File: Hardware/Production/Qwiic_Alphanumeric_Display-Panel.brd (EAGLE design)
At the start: 240.5 x 155.4 mm, 1080 parts, among them J11 Vertical Qwiic Connector, J12 Vertical Qwiic Connector, J14 Vertical Qwiic Connector, J15 Vertical Qwiic Connector, J17 Vertical Qwiic Connector, J18 Vertical Qwiic Connector, J2 Vertical Qwiic Connector, J20 Vertical Qwiic Connector, J21 Vertical Qwiic Connector, J23 Vertical Qwiic Connector, J24 Vertical Qwiic Connector, J26 Vertical Qwiic Connector, J27 Vertical Qwiic Connector, J29 Vertical Qwiic Connector, J30 Vertical Qwiic Connector, J32 Vertical Qwiic Connector, J33 Vertical Qwiic Connector, J35 Vertical Qwiic Connector, J36 Vertical Qwiic Connector, J38 Vertical Qwiic Connector, J39 Vertical Qwiic Connector, J4 Vertical Qwiic Connector, J41 Vertical Qwiic Connector, J42 Vertical Qwiic Connector, J44 Vertical Qwiic Connector, J45 Vertical Qwiic Connector, J47 Vertical Qwiic Connector, J48 Vertical Qwiic Connector, J5 Vertical Qwiic Connector, J50 Vertical Qwiic Connector, J51 Vertical Qwiic Connector, J53 Vertical Qwiic Connector, J54 Vertical Qwiic Connector, J56 Vertical Qwiic Connector, J57 Vertical Qwiic Connector, J59 Vertical Qwiic Connector, J6 Vertical Qwiic Connector, J60 Vertical Qwiic Connector, J62 Vertical Qwiic Connector, J63 Vertical Qwiic Connector, J65 Vertical Qwiic Connector, J66 Vertical Qwiic Connector, J68 Vertical Qwiic Connector, J69 Vertical Qwiic Connector, J71 Vertical Qwiic Connector, J72 Vertical Qwiic Connector, J74 Vertical Qwiic Connector, J75 Vertical Qwiic Connector, J8 Vertical Qwiic Connector, J9 Vertical Qwiic Connector

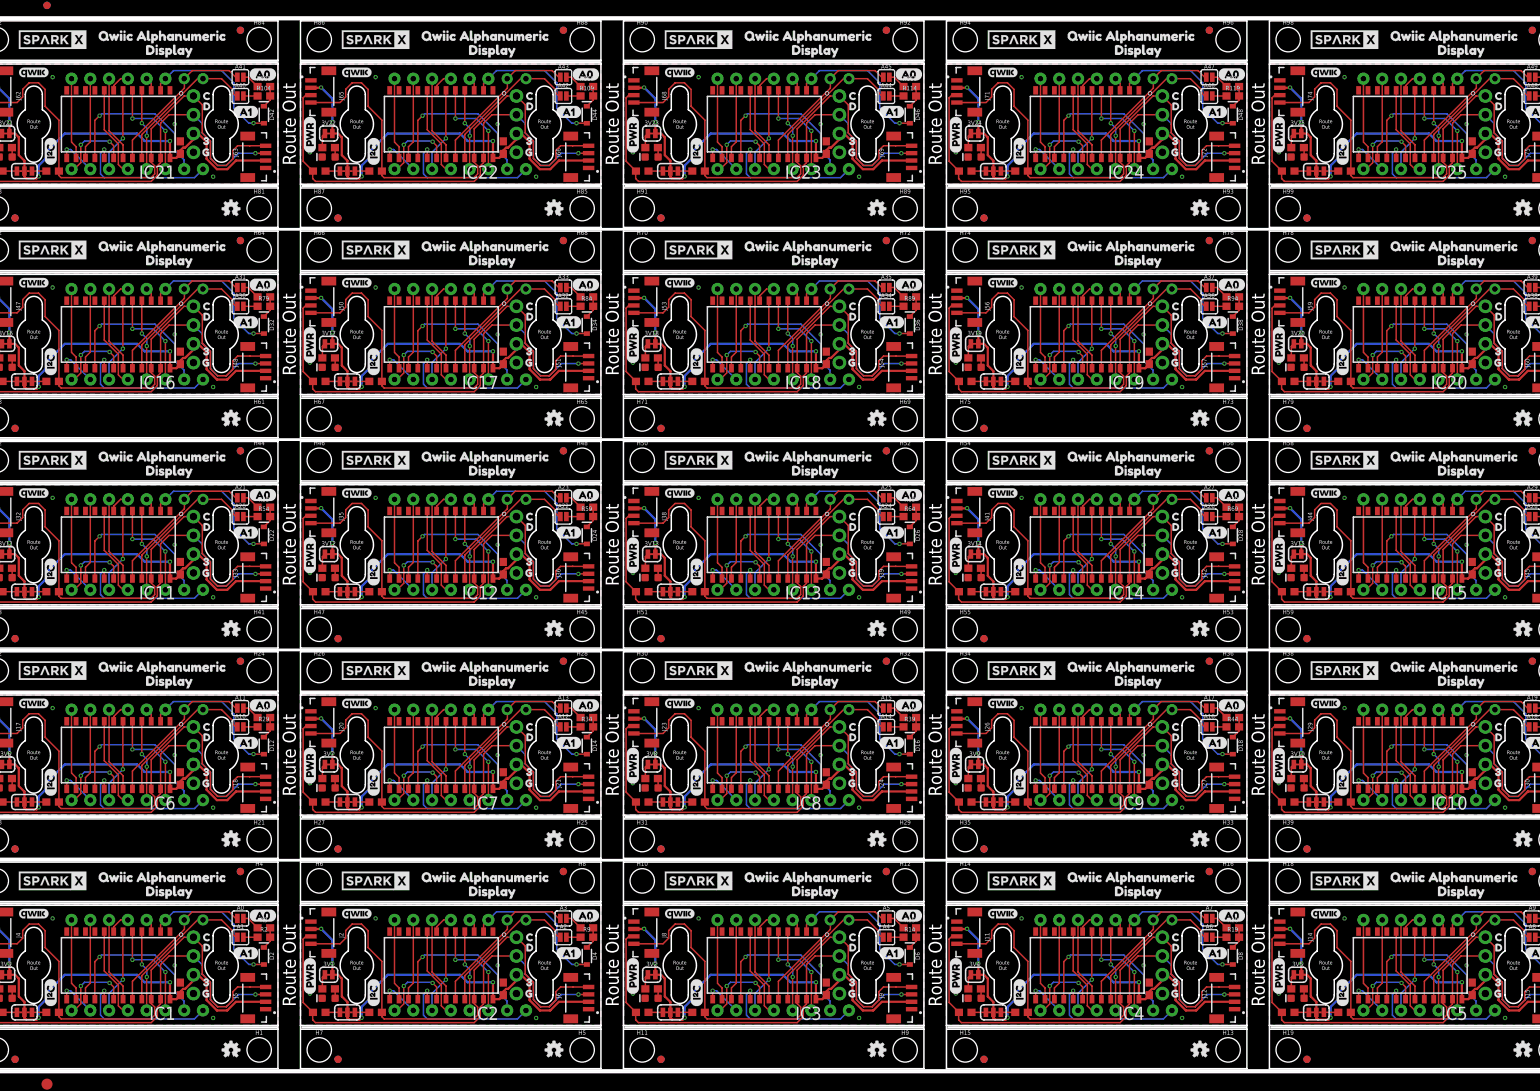
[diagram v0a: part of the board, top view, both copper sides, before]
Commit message: Added extra decoupling cap
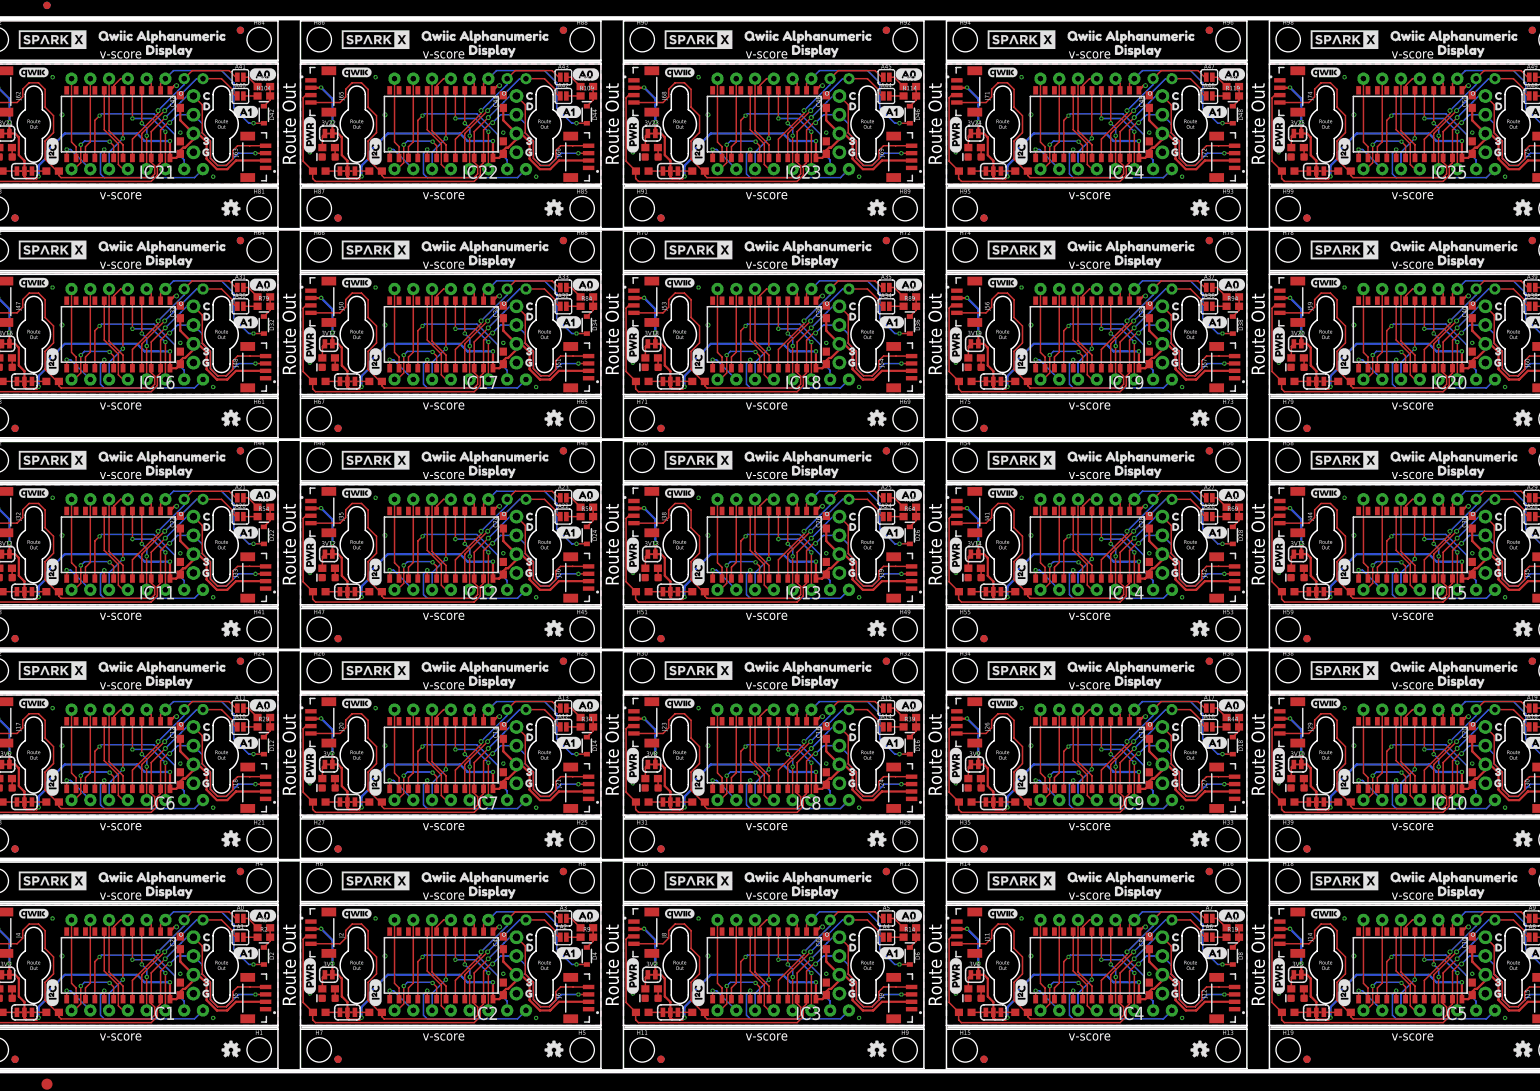
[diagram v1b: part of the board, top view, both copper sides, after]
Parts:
- added C26, C28, C30, C32, C34, C36, C38, C40, C42, C44, C46, C48, C50: 10uF, SparkFun-Capacitors:0603
- added C27, C29, C31, C33, C35, C37, C39, C41, C43, C45, C47, C49: 0.1uF, SparkFun-Capacitors:0603
- C1, C11, C13, C15, C17, C19, C21, C23, C25, C3, C5, C7, C9: value 1.0uF -> 0.1uF
- C10, C12, C14, C16, C18, C2, C20, C22, C24, C4, C6, C8: value 1.0uF -> 10uF
- moved C17 104.3 mm to (158.5, 39.2)
- moved C25 104.3 mm to (114.8, 67.7)
- moved C16 101.0 mm to (114.8, 45.5)
- moved C24 101.0 mm to (71.1, 73.9)
- moved C7 91.9 mm to (158.5, 10.8)
- moved C15 91.9 mm to (114.8, 39.2)
- moved C14 90.2 mm to (71.1, 45.5)
- moved C6 90.2 mm to (114.8, 17.0)
- moved C4 87.6 mm to (71.1, 17.0)
- moved C5 87.4 mm to (114.8, 10.8)
- moved C23 71.7 mm to (71.1, 67.7)
- moved C19 71.7 mm to (202.2, 39.2)
- moved C18 66.9 mm to (158.5, 45.5)
- moved C22 66.9 mm to (27.4, 73.9)
- moved C21 56.9 mm to (27.4, 67.7)
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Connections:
- net 3.3V: now also C2.1
- net 3.3V1: now also C3.1, C4.1; no longer C2.1
- net 3.3V10: now also C21.1, C22.1; no longer C11.1
- net 3.3V11: now also C23.1, C24.1; no longer C12.1
- net 3.3V12: now also C25.1, C26.1; no longer C13.1
- net 3.3V13: now also C27.1, C28.1; no longer C14.1
- net 3.3V14: now also C29.1, C30.1; no longer C15.1
- net 3.3V15: now also C31.1, C32.1; no longer C16.1
- net 3.3V16: now also C33.1, C34.1; no longer C17.1
- net 3.3V17: now also C35.1, C36.1; no longer C18.1
- net 3.3V18: now also C37.1, C38.1; no longer C19.1
- net 3.3V19: now also C39.1, C40.1; no longer C20.1
- net 3.3V2: now also C5.1, C6.1; no longer C3.1
- net 3.3V20: now also C41.1, C42.1; no longer C21.1
- net 3.3V21: now also C43.1, C44.1; no longer C22.1
- net 3.3V22: now also C45.1, C46.1; no longer C23.1
- net 3.3V23: now also C47.1, C48.1; no longer C24.1
- net 3.3V24: now also C49.1, C50.1; no longer C25.1
- net 3.3V3: now also C7.1, C8.1; no longer C4.1
- net 3.3V4: now also C10.1, C9.1; no longer C5.1
- net 3.3V5: now also C11.1, C12.1; no longer C6.1
- net 3.3V6: now also C13.1, C14.1; no longer C7.1
- net 3.3V7: now also C15.1, C16.1; no longer C8.1
- net 3.3V8: now also C17.1, C18.1; no longer C9.1
- net 3.3V9: now also C19.1, C20.1; no longer C10.1
- net GND: now also C2.2
- net GND1: now also C3.2, C4.2; no longer C2.2
- net GND10: now also C21.2, C22.2; no longer C11.2
- net GND11: now also C23.2, C24.2; no longer C12.2
- net GND12: now also C25.2, C26.2; no longer C13.2
- net GND13: now also C27.2, C28.2; no longer C14.2
- net GND14: now also C29.2, C30.2; no longer C15.2
- net GND15: now also C31.2, C32.2; no longer C16.2
- net GND16: now also C33.2, C34.2; no longer C17.2
- net GND17: now also C35.2, C36.2; no longer C18.2
- net GND18: now also C37.2, C38.2; no longer C19.2
- net GND19: now also C39.2, C40.2; no longer C20.2
- net GND2: now also C5.2, C6.2; no longer C3.2
- net GND20: now also C41.2, C42.2; no longer C21.2
- net GND21: now also C43.2, C44.2; no longer C22.2
- net GND22: now also C45.2, C46.2; no longer C23.2
- net GND23: now also C47.2, C48.2; no longer C24.2
- net GND24: now also C49.2, C50.2; no longer C25.2
- net GND3: now also C7.2, C8.2; no longer C4.2
- net GND4: now also C10.2, C9.2; no longer C5.2
- net GND5: now also C11.2, C12.2; no longer C6.2
- net GND6: now also C13.2, C14.2; no longer C7.2
- net GND7: now also C15.2, C16.2; no longer C8.2
- net GND8: now also C17.2, C18.2; no longer C9.2
- net GND9: now also C19.2, C20.2; no longer C10.2
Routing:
- net 3.3V19: track 60.6 -> 64.8 mm
- net 3.3V17: track 60.6 -> 64.8 mm
- net 3.3V15: track 60.6 -> 64.8 mm
- net 3.3V: track 60.6 -> 64.8 mm
- net 3.3V8: track 60.6 -> 64.8 mm
- net 3.3V7: track 60.6 -> 64.8 mm
- net 3.3V6: track 60.6 -> 64.8 mm
- net 3.3V5: track 60.6 -> 64.8 mm
- net 3.3V3: track 60.6 -> 64.8 mm
- net 3.3V23: track 60.6 -> 64.8 mm
- net 3.3V22: track 60.6 -> 64.8 mm
- net 3.3V21: track 60.6 -> 64.8 mm
- net 3.3V20: track 60.6 -> 64.8 mm
- net 3.3V2: track 60.6 -> 64.8 mm
- net 3.3V16: track 60.6 -> 64.8 mm
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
